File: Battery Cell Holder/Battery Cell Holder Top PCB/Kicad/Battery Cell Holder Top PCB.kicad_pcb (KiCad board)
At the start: 2 copper layers, 39 x 70 mm, 10 parts

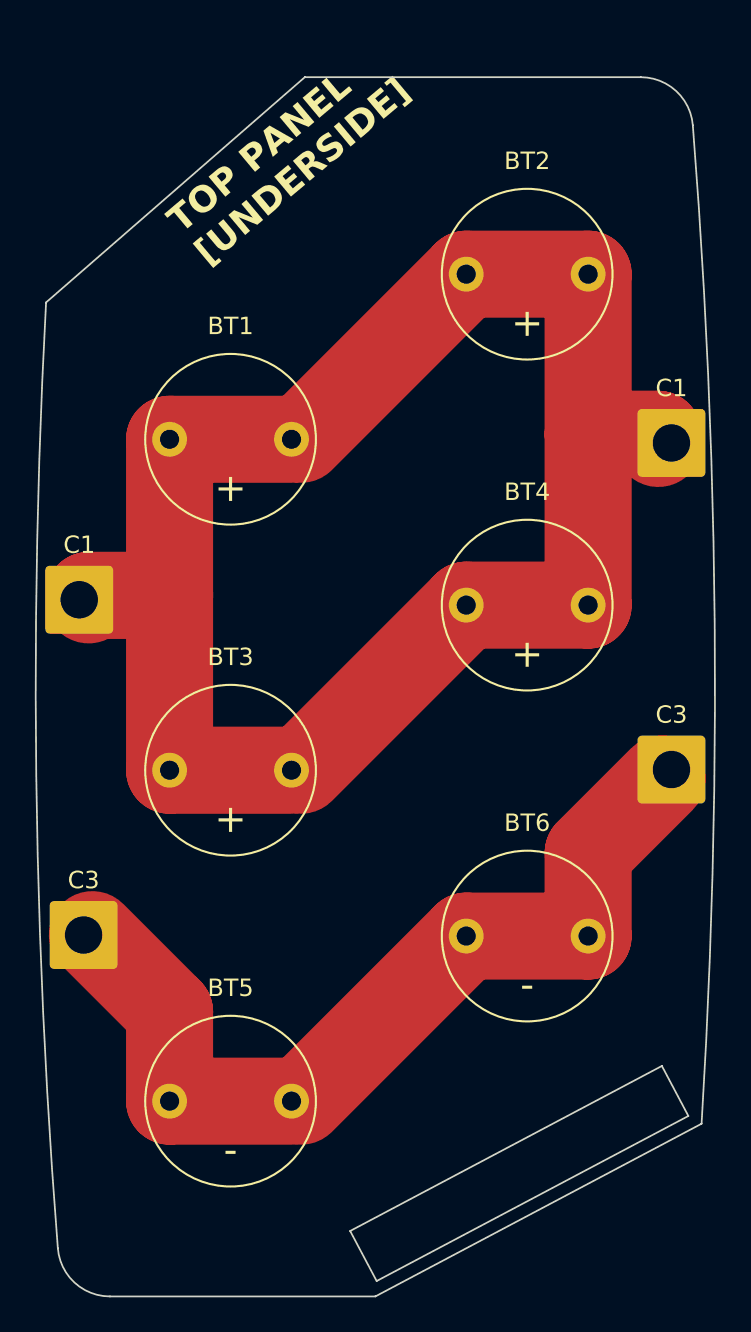
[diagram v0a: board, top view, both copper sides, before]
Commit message: fixes to boards
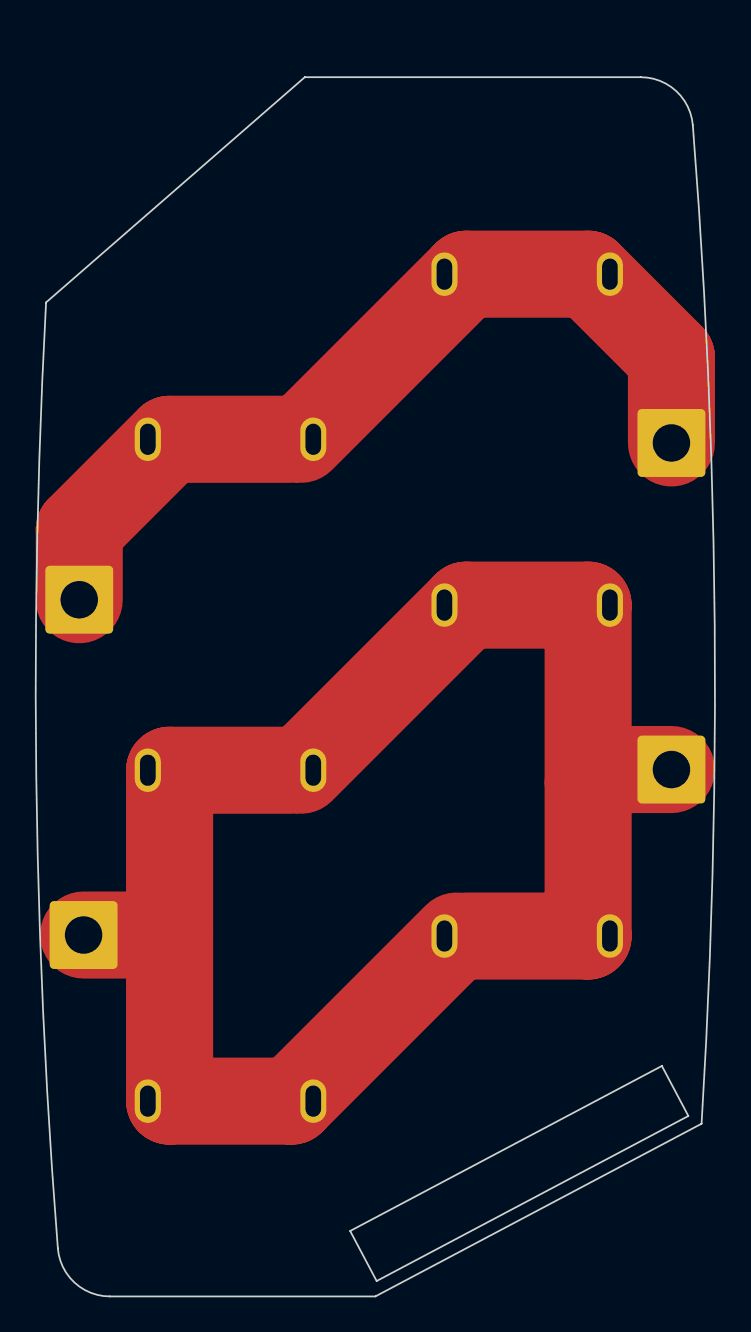
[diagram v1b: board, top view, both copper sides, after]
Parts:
- 12.6V: renamed from C1; moved to B.Cu
- 12.6V: renamed from BT1; footprint BatterySpringContact:Keystone_5222_SpringContact_THM -> C19724688:TH-2_BD10.0_F10-12-0.5-1.3UU-SUS304; moved to B.Cu
- 12.6V: renamed from BT2; footprint BatterySpringContact:Keystone_5222_SpringContact_THM -> C19724688:TH-2_BD10.0_F10-12-0.5-1.3UU-SUS304; moved to B.Cu
- 4.2V: renamed from BT5; footprint BatterySpringContact:Keystone_5222_SpringContact_THM -> C19724688:TH-2_BD10.0_F10-12-0.5-1.3UU-SUS304; moved to B.Cu
- 4.2V: renamed from BT6; footprint BatterySpringContact:Keystone_5222_SpringContact_THM -> C19724688:TH-2_BD10.0_F10-12-0.5-1.3UU-SUS304; moved to B.Cu
- 8.4V: renamed from BT3; footprint BatterySpringContact:Keystone_5222_SpringContact_THM -> C19724688:TH-2_BD10.0_F10-12-0.5-1.3UU-SUS304; moved to B.Cu
- 8.4V: renamed from BT4; footprint BatterySpringContact:Keystone_5222_SpringContact_THM -> C19724688:TH-2_BD10.0_F10-12-0.5-1.3UU-SUS304; moved to B.Cu
- turned 12.6V to 180 degrees (x3)
- turned 4.2V to 180 degrees (x2)
- turned 8.4V to 180 degrees (x2)
- renumbered C1 to 12.6V, C3 to 8.4V
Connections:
- 12.6V pad 1: /C1 -> /C3 (x4)
- 4.2V pad 1: /C3 -> /C2 (x2)
- 8.4V pad 1: /C3 -> /C2 (x2)
- 8.4V pad 1: /C1 -> /C2 (x2)
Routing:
- net /C2: track 0.00 -> 104.6 mm
- net /C1: track 103.4 -> 0.00 mm
- net /C3: track 50.1 -> 51.0 mm
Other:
- board text added: "+"
- board text added: "-"
- board text added: "12.6V"
- board text added: "4.2V"
- board text added: "TOP PANEL [UNDER SIDE]"
- board text removed: "TOP PANEL [UNDERSIDE]"
